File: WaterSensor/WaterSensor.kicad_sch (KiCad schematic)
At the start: 9 parts, among them J1 Conn_02x07_Odd_Even, J2 USB_B_Micro, U13 CH340E

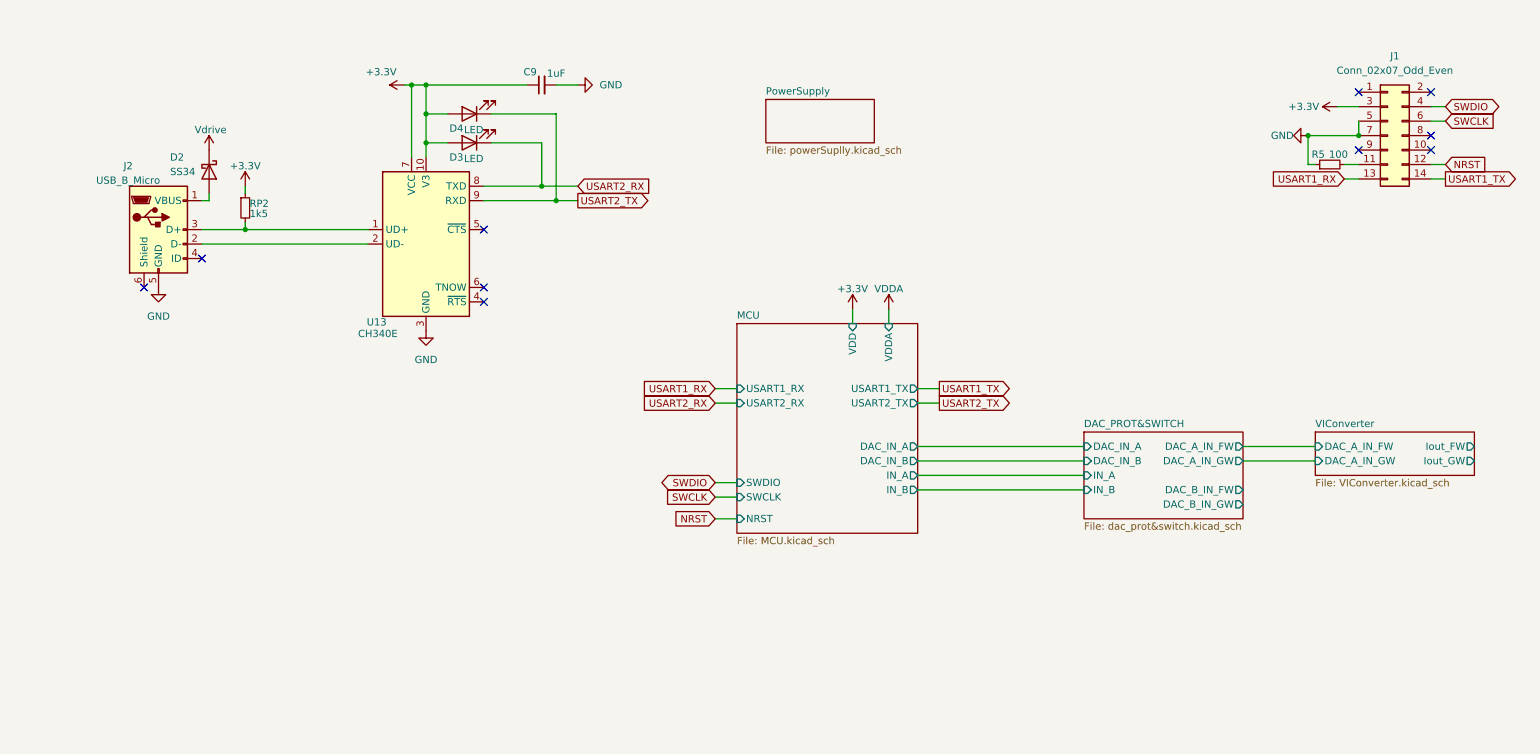
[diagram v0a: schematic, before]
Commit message: schematic done
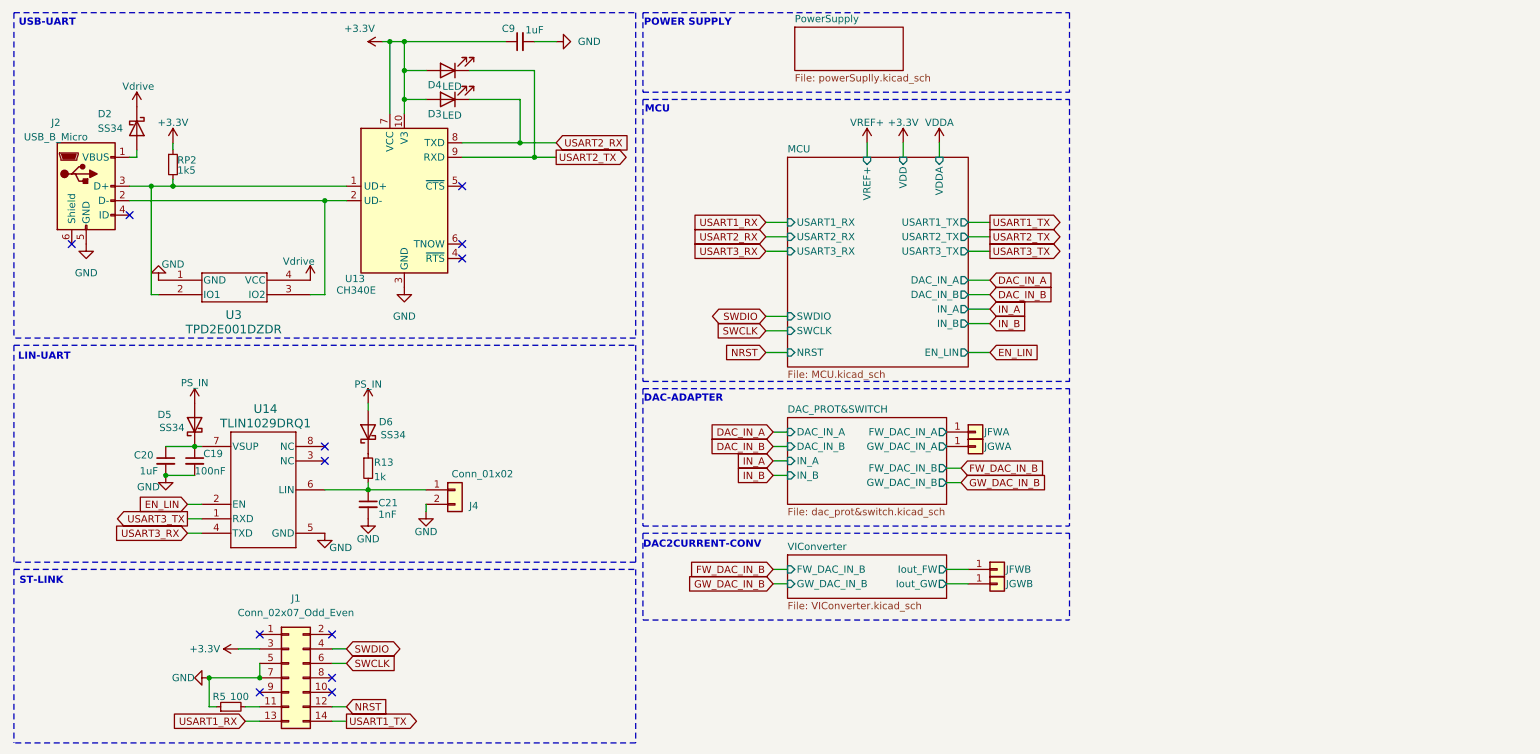
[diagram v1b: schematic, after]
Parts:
- added C19: 100nF, symbol Device:C_Small
- added C20: 1uF, symbol Device:C_Small
- added C21: 1nF, symbol Device:C_Small
- added D5, D6: SS34, Diode_SMD:D_SMA, symbol Diode:SS34
- added J4: Conn_01x02, symbol Connector_Generic:Conn_01x02
- added JFWA, JFWB, JGWA, JGWB: ~, symbol Connector_Generic:Conn_01x01
- added R13: 1k, symbol Device:R_Small
- added U14: TLIN1029DRQ1, D0008A_N, symbol TLIN1029DRQ1:TLIN1029DRQ1
- added U3: TPD2E001DZDR, DZD4, symbol TPD2E001DZDR:TPD2E001DZDR
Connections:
- net GND: now also C19.2, C20.2, C21.2, J4.2 (Pin_2), U14.5 (GND), U3.1 (GND)
- net VIConverter/Iout_FW: now also JFWB.1 (Pin_1)
- net VIConverter/Iout_GW: now also JGWB.1 (Pin_1)
- net Vdrive: now also U3.4 (VCC)
- net at J2.2 (D-), U13.2 (UD-): now also U3.3 (IO2)
- net at J2.3 (D+), RP2.2, U13.1 (UD+): now also U3.2 (IO1)
- new net: D6.1 (K), R13.1
- new net: C21.1, J4.1 (Pin_1), R13.2, U14.6 (LIN)
- new net: C19.1, C20.1, D5.1 (K), U14.7 (VSUP)
- new net DAC_PROT&SWITCH/FW_DAC_IN_A: JFWA.1 (Pin_1)
- new net DAC_PROT&SWITCH/GW_DAC_IN_A: JGWA.1 (Pin_1)
- new net EN_LIN: U14.2 (EN)
- new net PS_IN: D5.2 (A), D6.2 (A)
- new net USART3_RX: U14.4 (TXD)
- new net USART3_TX: U14.1 (RXD)
- no-connect marks 10 -> 12
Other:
- sheet DAC_PROT&SWITCH ports: added FW_DAC_IN_A, FW_DAC_IN_B, GW_DAC_IN_A, GW_DAC_IN_B; removed DAC_A_IN_FW, DAC_A_IN_GW, DAC_B_IN_FW, DAC_B_IN_GW
- sheet MCU ports: added EN_LIN, USART3_RX, USART3_TX, VREF+; removed none
- sheet VIConverter ports: added FW_DAC_IN_B, GW_DAC_IN_B; removed DAC_A_IN_FW, DAC_A_IN_GW
- note added: "DAC-ADAPTER"
- note added: "DAC2CURRENT-CONV"
- note added: "LIN-UART"
- note added: "MCU"
- note added: "POWER SUPPLY"
- note added: "ST-LINK"
- note added: "USB-UART"
- moved on the sheet: C9, D2, D3, D4, J1, J2, R5, RP2, U13
